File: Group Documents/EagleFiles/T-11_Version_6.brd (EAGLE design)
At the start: 100 x 80 mm, 52 parts, among them SW1 SW-1801X, SW2 SW-1801X, U1 ATMEGA328P-AU, X1 SMA-142-0701-871/880

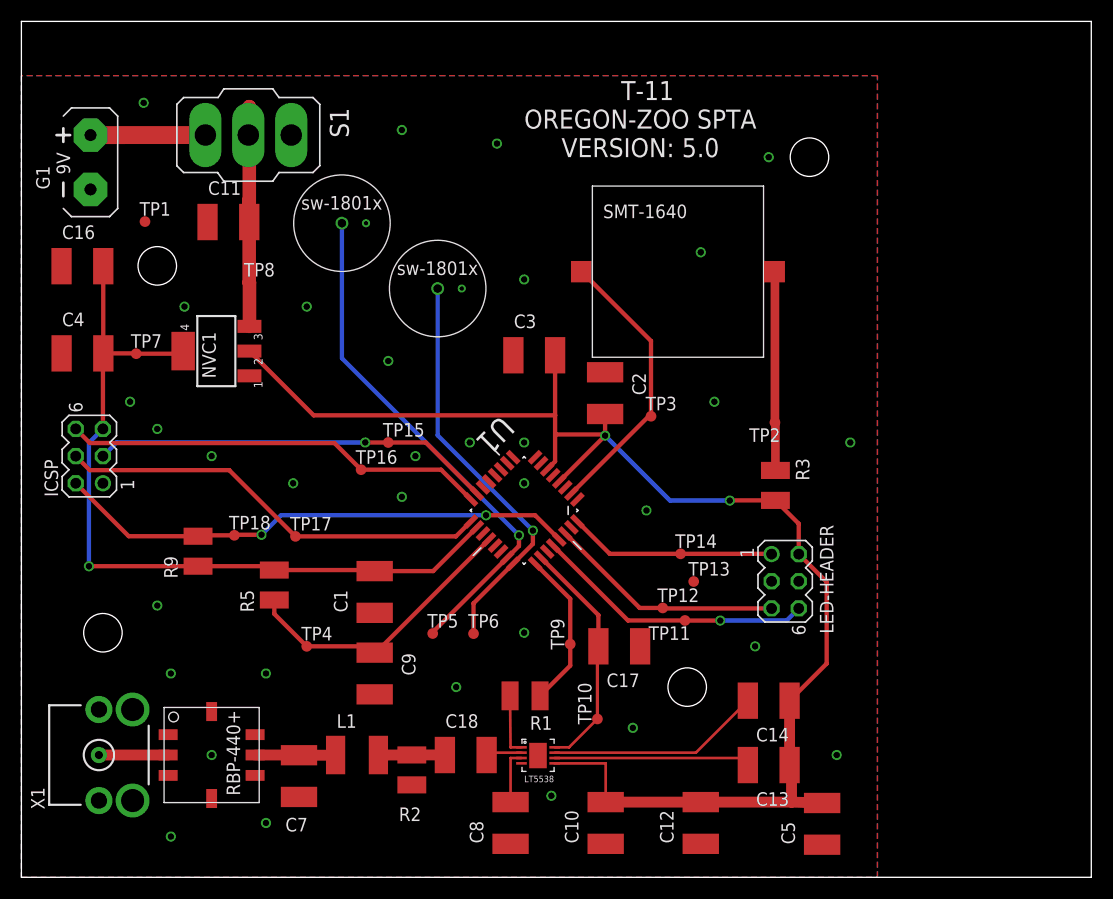
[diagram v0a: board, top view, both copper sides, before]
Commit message: T-11 SPTA_V6-update
Updated Read_me
updated schematic
updated board layout
Updated BOM
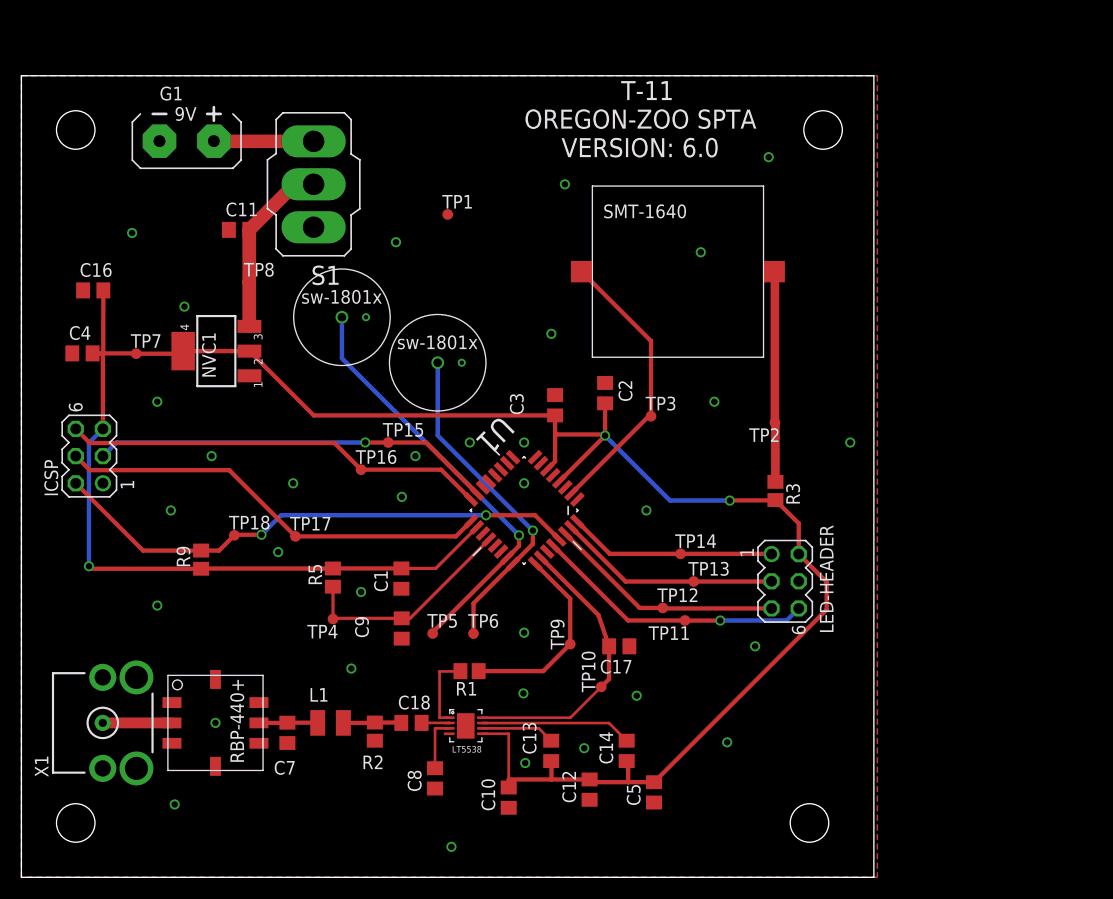
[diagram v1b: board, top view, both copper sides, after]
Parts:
- C1, C10, C11, C12, C13, C14, C16, C17, C18, C2, C3, C4, C5, C7, C8, C9: device rcl:C4532 -> rcl:C0805
- L1: device rcl:L4532P -> resistor:L2825P
- R1, R2, R3, R5, R9: device rcl:R3225 -> resistor:R0805
- S1: value POWER_SW -> (none)
- moved TP1 28.3 mm to (39.8, 62.0)
- moved C13 20.4 mm to (49.5, 11.8), turned to 90 degrees
- moved C5 16.0 mm to (59.1, 7.94)
- moved C14 14.1 mm to (56.6, 11.8), turned to 90 degrees
- moved C12 10.8 mm to (53.1, 8.20)
- moved C10 9.37 mm to (45.5, 7.45)
- moved G1 9.21 mm to (15.5, 68.8), turned to 270 degrees
- moved SW1 8.79 mm to (30.0, 52.3)
- moved C8 8.20 mm to (38.7, 9.25)
- moved S1 7.65 mm to (27.3, 64.8), turned to 180 degrees
- moved LT5538 7.30 mm to (41.5, 14.2)
- moved SW2 6.93 mm to (38.9, 48.1)
- moved C18 5.90 mm to (36.5, 14.4)
- moved R1 5.68 mm to (41.9, 19.3)
- moved R5 5.52 mm to (29.1, 28.0)
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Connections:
- net N$7 renamed INDICATOR_2
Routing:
- net INDICATOR_2: track 0.00 -> 20.8 mm
- net N$9: track 18.7 -> 6.90 mm
- net PS_VIN: track 27.3 -> 16.8 mm
- net VIB_2: track 48.5 -> 39.8 mm
- net VIB_1: track 38.2 -> 31.3 mm
- net N$10: track 27.2 -> 20.7 mm
- net N$8: track 20.1 -> 14.2 mm
- net RF_OUT: track 22.4 -> 27.1 mm
- net RF_ENABLE: track 14.9 -> 18.5 mm
- net +5V: track 207.8 -> 210.6 mm
- net N$4: track 10.7 -> 9.33 mm
- net N$6: track 5.83 -> 7.21 mm
- net N$5: track 3.87 -> 2.59 mm
- net RESET: track 49.0 -> 50.1 mm
- net N$3: track 18.6 -> 19.7 mm
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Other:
- board size 100 x 80 mm -> 79.7 x 74.9 mm
- board text added: "T-11 OREGON-ZOO SPTA VERSION: 6.0"
- board text removed: "T-11 OREGON-ZOO SPTA VERSION: 5.0"
